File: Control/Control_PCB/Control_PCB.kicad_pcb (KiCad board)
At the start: 2 copper layers, 210 x 105 mm, 121 parts, among them J1 Motor_cont2, J10 NC, J11 IOREF, J12 RESET, J13 +3V3, J14 +5V_1, J15 GND1, J16 GND2, J17 VIN, J18 AD0, J19 AD1, J2 Motor_cont1, J20 AD2, J21 AD3, J22 AD4, J23 AD5, J24 AD6, J25 AD7, J26 AD8, J27 AD9, J28 AD10, J29 AD11, J3 Driver1, J30 AD12, J31 AD13, J32 AD14, J33 AD15, J34 +5V_3, J35 23, J36 25, J37 27, J38 29, J39 31, J4 ARM, J40 33, J41 35, J42 37, J43 39, J44 41, J45 43, J46 45, J47 47, J48 49, J49 51, J5 Encoder2, J50 53, J51 GND5, J52 SCL, J53 SDA, J54 AREF, J55 GND3, J56 13, J57 12, J58 11, J59 10, J6 Encoder1, J60 9, J61 8, J62 7, J63 6, J64 5, J65 4, J66 3, J67 2, J68 1, J69 0, J7 Router_Power, J70 21, J71 20, J72 19, J73 18, J74 17, J75 16, J76 15, J77 14, J78 +5V_2, J79 22, J8 Metal_Sensor, J80 24, J81 26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

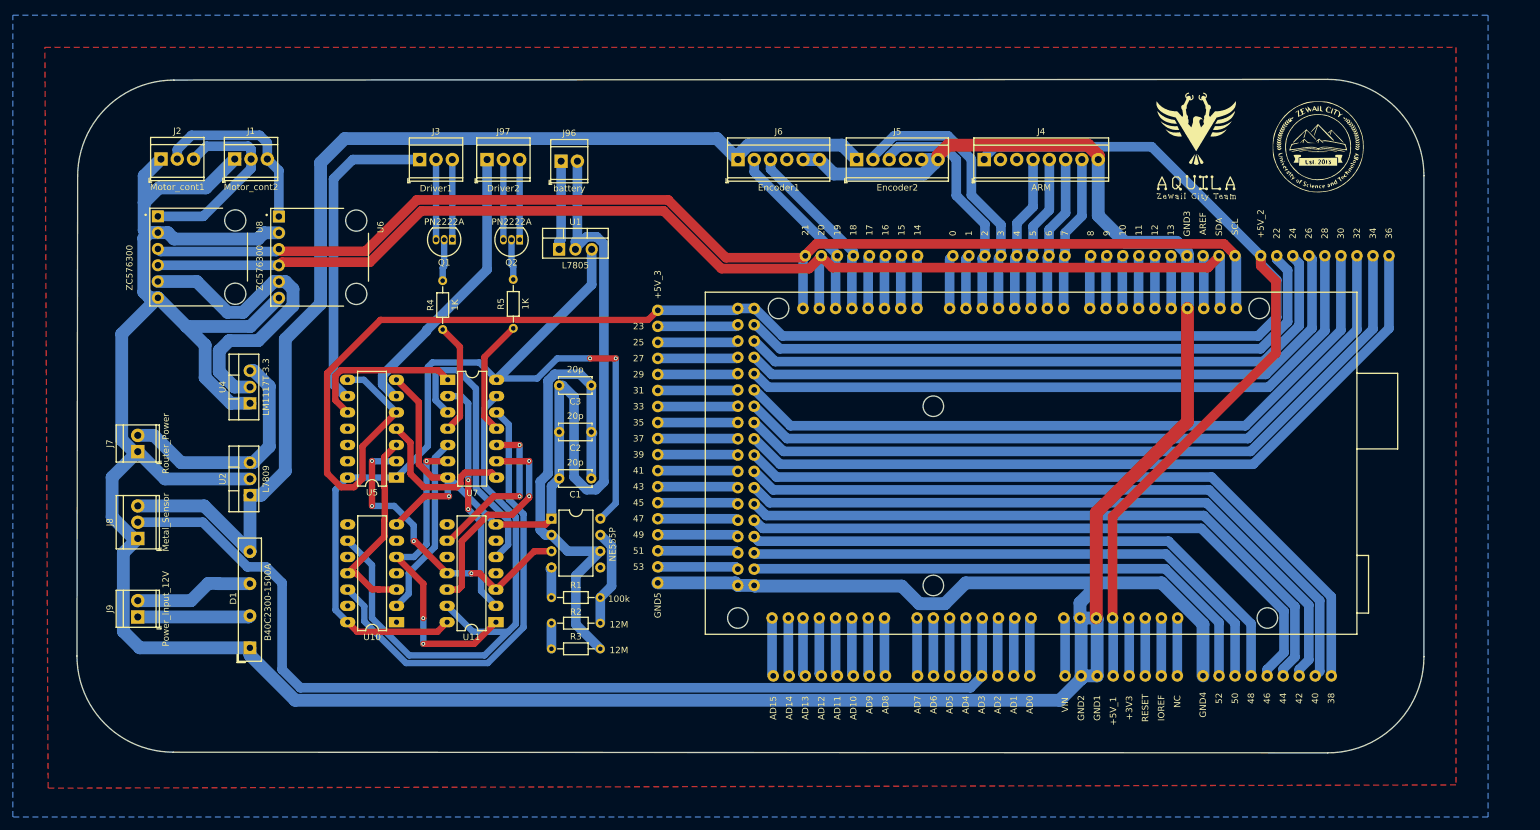
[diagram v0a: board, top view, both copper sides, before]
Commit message: Second commit
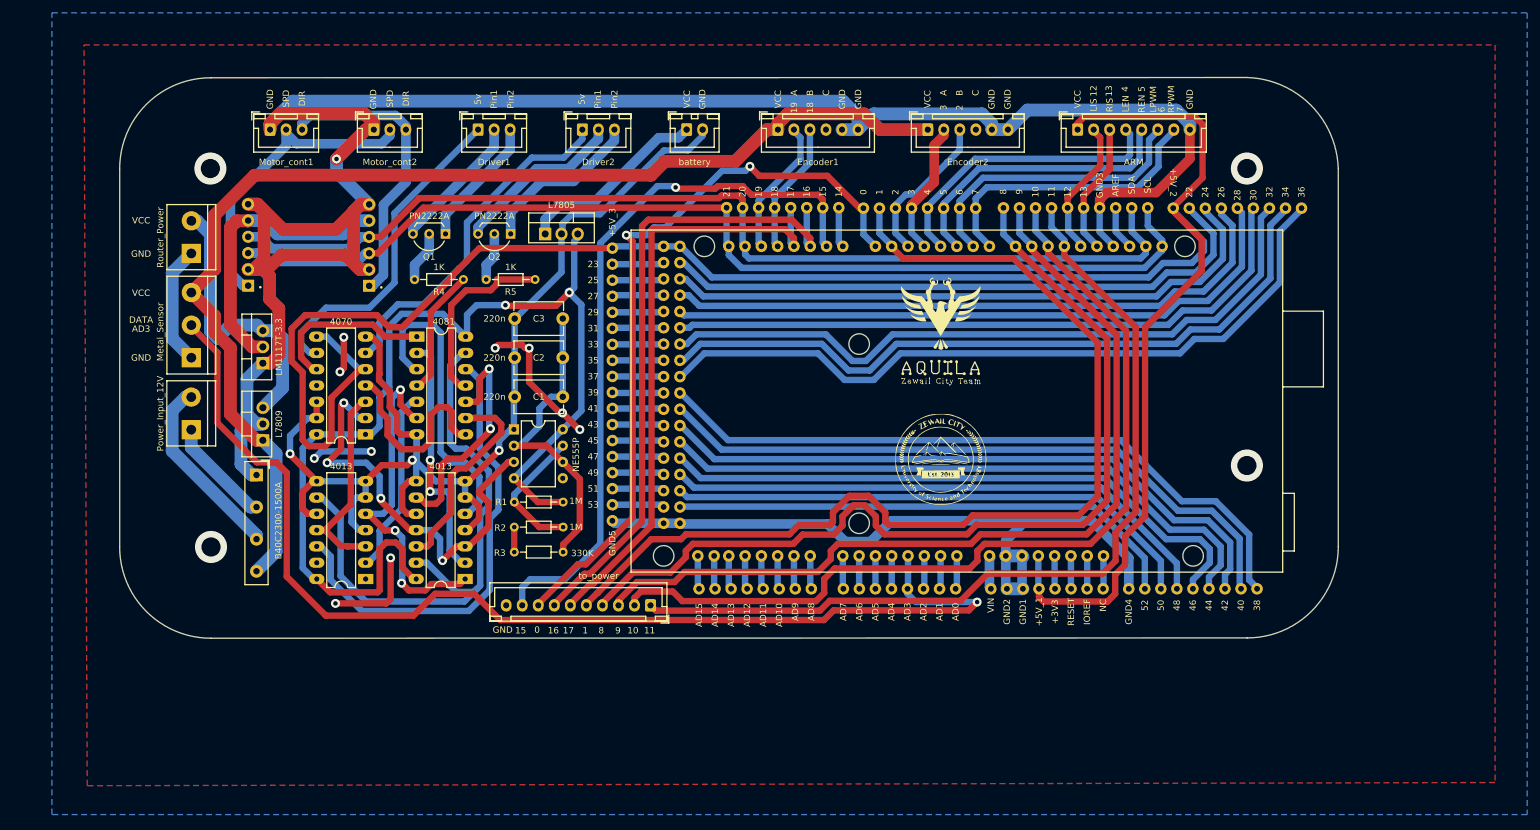
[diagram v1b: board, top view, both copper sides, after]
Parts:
- added J98: to_power, Connector_JST:JST_XH_B10B-XH-A_1x10_P2.50mm_Vertical, F.Cu at (124.4, 127.0)
- C1, C2, C3: value 20p -> 220n; footprint Capacitor_THT:C_Disc_D5.0mm_W2.5mm_P5.00mm -> Capacitor_THT:C_Disc_D7.5mm_W5.0mm_P7.50mm
- J1, J2, J3, J97: footprint TerminalBlock_TE-Connectivity:TerminalBlock_TE_282834-3_1x03_P2.54mm_Horizontal -> Connector_JST:JST_XH_B3B-XH-A_1x03_P2.50mm_Vertical
- J4: footprint TerminalBlock_TE-Connectivity:TerminalBlock_TE_282834-8_1x08_P2.54mm_Horizontal -> Connector_JST:JST_XH_B8B-XH-A_1x08_P2.50mm_Vertical
- J5, J6: footprint TerminalBlock_TE-Connectivity:TerminalBlock_TE_282834-6_1x06_P2.54mm_Horizontal -> Connector_JST:JST_XH_B6B-XH-A_1x06_P2.50mm_Vertical
- J7, J9: footprint TerminalBlock_TE-Connectivity:TerminalBlock_TE_282834-2_1x02_P2.54mm_Horizontal -> MyLibrary:TerminalBlock_bornier-2_P5.08mm
- J8: footprint TerminalBlock_TE-Connectivity:TerminalBlock_TE_282834-3_1x03_P2.54mm_Horizontal -> MyLibrary:TerminalBlock_bornier-3_P5.08mm
- J96: footprint TerminalBlock_TE-Connectivity:TerminalBlock_TE_282834-2_1x02_P2.54mm_Horizontal -> Connector_JST:JST_XH_B2B-XH-A_1x02_P2.50mm_Vertical
- Q1, Q2: footprint Package_TO_SOT_THT:TO-92_Inline -> Package_TO_SOT_THT:TO-92L_Inline_Wide
- R1: value 100k -> 1M
- R2: value 12M -> 1M
- R3: value 12M -> 330K
- U6, U8: footprint External_footprint_lib:MODULE_ZC576300 -> MyLibrary:MODULE_ZC576300
- moved G*** 76.4 mm to (169.7, 104.2)
- moved G*** 49.2 mm to (169.7, 84.3)
- moved J7 32.0 mm to (52.8, 72.1)
- moved J9 30.4 mm to (52.8, 99.6)
- moved J8 29.4 mm to (52.8, 88.4)
- moved D1 27.0 mm to (63.0, 106.7), turned to -90 degrees
- moved J1 22.2 mm to (81.3, 52.8)
- moved J96 20.2 mm to (130.0, 52.8)
- moved J10 17.8 mm to (195.0, 124.4)
- moved J11 17.8 mm to (192.5, 124.4)
- moved J12 17.8 mm to (190.0, 124.4)
- moved J13 17.8 mm to (187.5, 124.4)
- moved J14 17.8 mm to (185.0, 124.4)
- moved J15 17.8 mm to (182.5, 124.4)
- moved J16 17.8 mm to (180.0, 124.4)
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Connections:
- net Net-(J58-Pin_1) renamed /11
- net Net-(J59-Pin_1) renamed /10
- net Net-(J60-Pin_1) renamed /9
- net Net-(J61-Pin_1) renamed /8
- net Net-(J68-Pin_1) renamed /1
- net Net-(J69-Pin_1) renamed /0
- net Net-(J74-Pin_1) renamed /17
- net Net-(J75-Pin_1) renamed /16
- net Net-(J76-Pin_1) renamed /15
- net Net-(J77-Pin_1) renamed /14
- A1 pad 12: Net-(J57-Pin_1) -> /LIS
- A1 pad 13: Net-(J56-Pin_1) -> /RIS
- J2 pad 2: /DAC2_Out -> /DAC1_Out
- J2 pad 3: /DAC1_Out -> /DAC2_Out
- J56 pad 1: Net-(J56-Pin_1) -> /RIS
- J57 pad 1: Net-(J57-Pin_1) -> /LIS
- R1 pad 1: /res_t -> /battery_vcc
- U10 pad 10: unconnected-(U10B-R-Pad10) -> /battery_gnd
- U10 pad 4: unconnected-(U10A-R-Pad4) -> /battery_gnd
- U10 pad 6: unconnected-(U10A-S-Pad6) -> /battery_gnd
- U10 pad 8: unconnected-(U10B-S-Pad8) -> /battery_gnd
- U11 pad 10: unconnected-(U11B-R-Pad10) -> /battery_gnd
- U11 pad 4: unconnected-(U11A-R-Pad4) -> /battery_gnd
- U11 pad 6: unconnected-(U11A-S-Pad6) -> /battery_gnd
- U11 pad 8: unconnected-(U11B-S-Pad8) -> /battery_gnd
- U5 pad 12: unconnected-(U5-Pad12) -> /battery_gnd
- U5 pad 13: unconnected-(U5-Pad13) -> /battery_gnd
- U9 pad 4: /res_t -> /battery_vcc
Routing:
- net /1: track 8.41 -> 161.4 mm
- net /8: track 8.28 -> 144.0 mm
- net /10: track 8.27 -> 139.7 mm
- net /9: track 8.26 -> 137.9 mm
- net /11: track 8.31 -> 137.9 mm
- net /0: track 8.42 -> 116.0 mm, vias 0 -> 2
- net /15: track 8.26 -> 111.8 mm, vias 0 -> 1
- net /16: track 8.28 -> 100.7 mm
- net GND: track 609.8 -> 519.3 mm, vias 0 -> 15
- net /17: track 8.30 -> 94.4 mm
- net /battery_gnd: track 152.1 -> 187.4 mm, vias 1 -> 3
- net /SCL: track 193.9 -> 163.2 mm
- net /SDA: track 191.8 -> 161.3 mm
- net /cap: track 75.5 -> 49.5 mm
- net /EN2_Phase_A: track 44.0 -> 21.1 mm
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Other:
- board size 210 x 105 mm -> 190 x 87.4 mm
- board text added: "0"
- board text added: "1"
- board text added: "10"
- board text added: "11"
- board text added: "12"
- board text added: "13"
- board text added: "15"
- board text added: "16"
- board text added: "17"
- board text added: "18"
- board text added: "19"
- board text added: "1M"
- board text added: "2"
- board text added: "3"
- board text added: "330K"
- board text added: "4"
- board text added: "5"
- board text added: "5v"
- board text added: "6"
- board text added: "7"
- board text added: "8"
- board text added: "9"
- board text added: "A"
- board text added: "AD3"
- board text added: "B"
- board text added: "C"
- board text added: "DATA"
- board text added: "DIR"
- board text added: "GND"
- board text added: "LEN"
- board text added: "LIS"
- board text added: "LPWM"
- board text added: "Pin1"
- board text added: "Pin2"
- board text added: "REN"
- board text added: "RIS"
- board text added: "RPWM"
- board text added: "SPD"
- board text added: "VCC"
- board text removed: "12M"
